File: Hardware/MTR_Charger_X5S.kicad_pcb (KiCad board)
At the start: 2 copper layers, 125 parts, among them J1 Korean Hroparts Elec TYPE-C-3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, J2 Micro_SD_Card, Q1 IRF7324TRPBF, Q10 AO3480C, Q11 AO3480C, Q2 AO3401A, Q3 AO3401A, Q4 AO3480C, Q5 AO3480C, Q6 AO3401A, Q7 AO3480C, Q8 AO3401A, Q9 AO3401A, SW1 Boot, SW2 Reset, U1 W25Q16JVUXIQ, U10 LMC6482AIMX/NOPB, U11 LMC6482AIMX/NOPB, U12 LMC6482AIMX/NOPB, U13 LMC6482AIMX/NOPB, U14 TCA9535PWR_C130204, U15 CD74HCT4051M96, U2 RP2040, U3 ADS7830IPWR, U4 ADS7830IPWR, U5 ESDA25W, U6 STUSB4500QTR, U7 MCP73833-AMI/MF, U8 LMV358IDR, U9 LMC6482AIMX/NOPB, X1 X322512MSB4SI

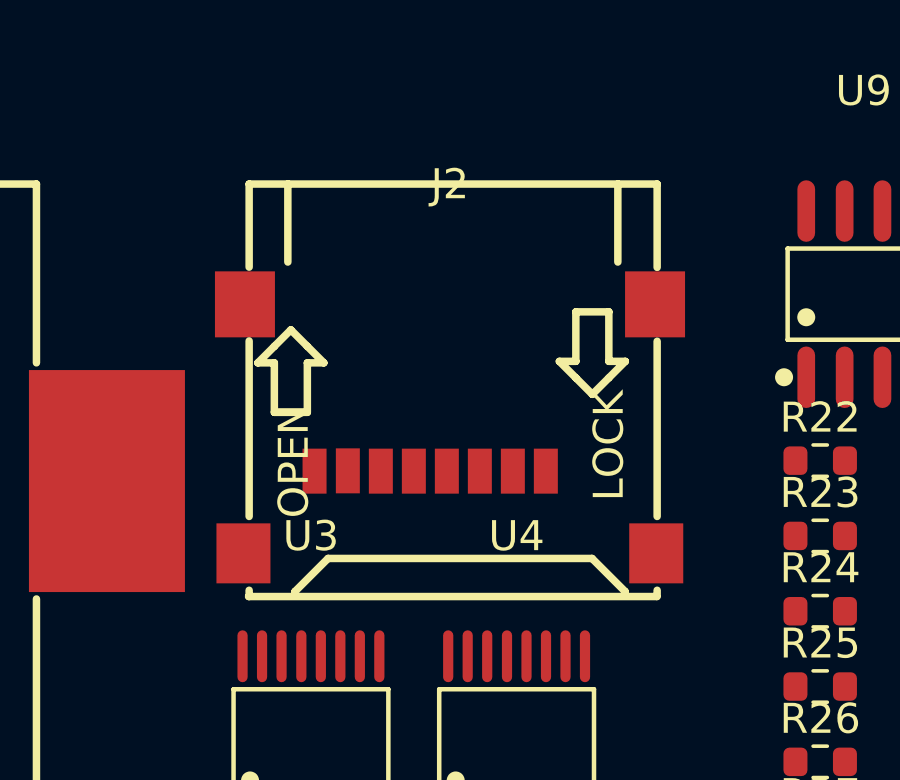
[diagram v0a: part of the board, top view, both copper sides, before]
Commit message: --------------
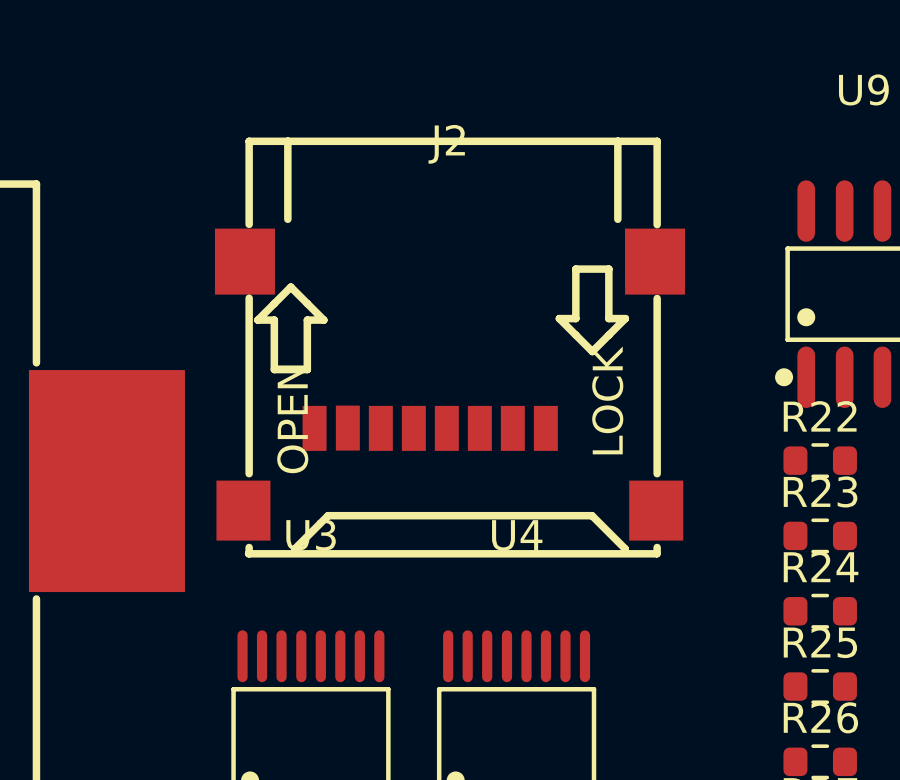
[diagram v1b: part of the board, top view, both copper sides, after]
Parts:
- moved J2 1.43 mm to (137.4, 49.0)
